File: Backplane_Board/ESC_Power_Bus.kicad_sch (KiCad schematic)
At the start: 18 parts, among them J5 Conn_01x02_Pin, SW1 SW_DPST_x2, U3 PKJ7213WPI

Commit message: derat nest ifcation
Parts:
- C10, C11, C12, C9: footprint C2012X5R1V226M125AC:CAPC2012X145N -> Capacitor_SMD:C_1206_3216Metric_Pad1.33x1.80mm_HandSolder
- R6: footprint Resistor_SMD:R_1206_3216Metric_Pad1.30x1.75mm_HandSolder -> Resistor_SMD:R_0805_2012Metric_Pad1.20x1.40mm_HandSolder
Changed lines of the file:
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@@
 			)
 		)
-		(property "Footprint" "C2012X5R1V226M125AC:CAPC2012X145N"
+		(property "Footprint" "Capacitor_SMD:C_1206_3216Metric_Pad1.33x1.80mm_HandSolder"
 			(at 243.84 139.7 0)
 			(effects
@@
 			)
 		)
-		(property "Footprint" "Resistor_SMD:R_1206_3216Metric_Pad1.30x1.75mm_HandSolder"
+		(property "Footprint" "Resistor_SMD:R_0805_2012Metric_Pad1.20x1.40mm_HandSolder"
 			(at 99.822 69.85 90)
 			(effects
@@
 			)
 		)
-		(property "Footprint" "C2012X5R1V226M125AC:CAPC2012X145N"
+		(property "Footprint" "Capacitor_SMD:C_1206_3216Metric_Pad1.33x1.80mm_HandSolder"
 			(at 204.47 139.7 0)
 			(effects
@@
 			)
 		)
-		(property "Footprint" "C2012X5R1V226M125AC:CAPC2012X145N"
+		(property "Footprint" "Capacitor_SMD:C_1206_3216Metric_Pad1.33x1.80mm_HandSolder"
 			(at 224.79 139.7 0)
 			(effects
@@
 			)
 		)
-		(property "Footprint" "C2012X5R1V226M125AC:CAPC2012X145N"
+		(property "Footprint" "Capacitor_SMD:C_1206_3216Metric_Pad1.33x1.80mm_HandSolder"
 			(at 186.69 139.7 0)
 			(effects

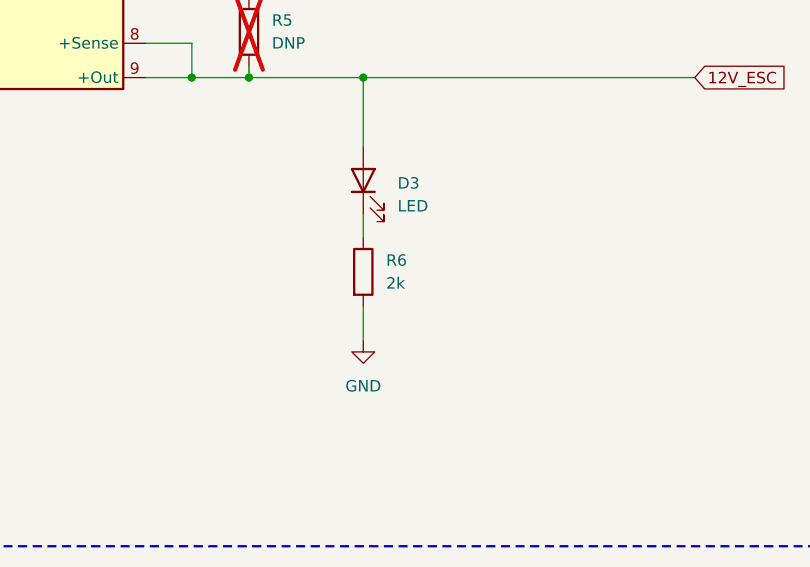
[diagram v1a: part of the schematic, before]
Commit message: added gerber
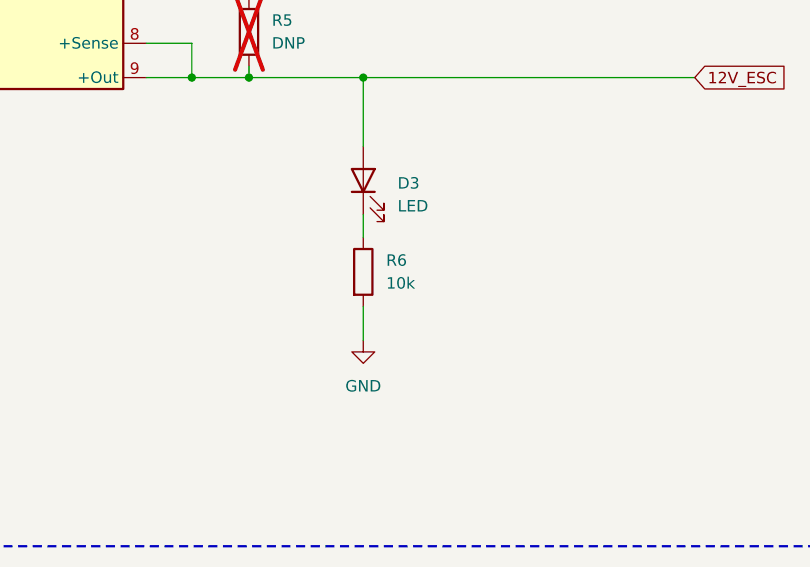
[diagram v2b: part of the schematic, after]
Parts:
- R6: value 2k -> 10k
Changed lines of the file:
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@@
 			)
 		)
-		(property "Value" "2k"
+		(property "Value" "10k"
 			(at 104.14 71.1199 0)
 			(effects
